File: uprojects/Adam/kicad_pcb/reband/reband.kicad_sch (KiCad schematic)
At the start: 32 parts, among them IC1 USBLC6-2SC6, J1 S2B-ZRLFSN, J2 USB4215-03-A, U1 ESP32-C3FH4, U2 TLV75533PDBVR, U3 MAX30009ENA+T, U4 BQ25100YFPR, U5 BNO055, U7 TCR2EF18_LMCT, Y1 ECS-400-18-33-JGN-TR3

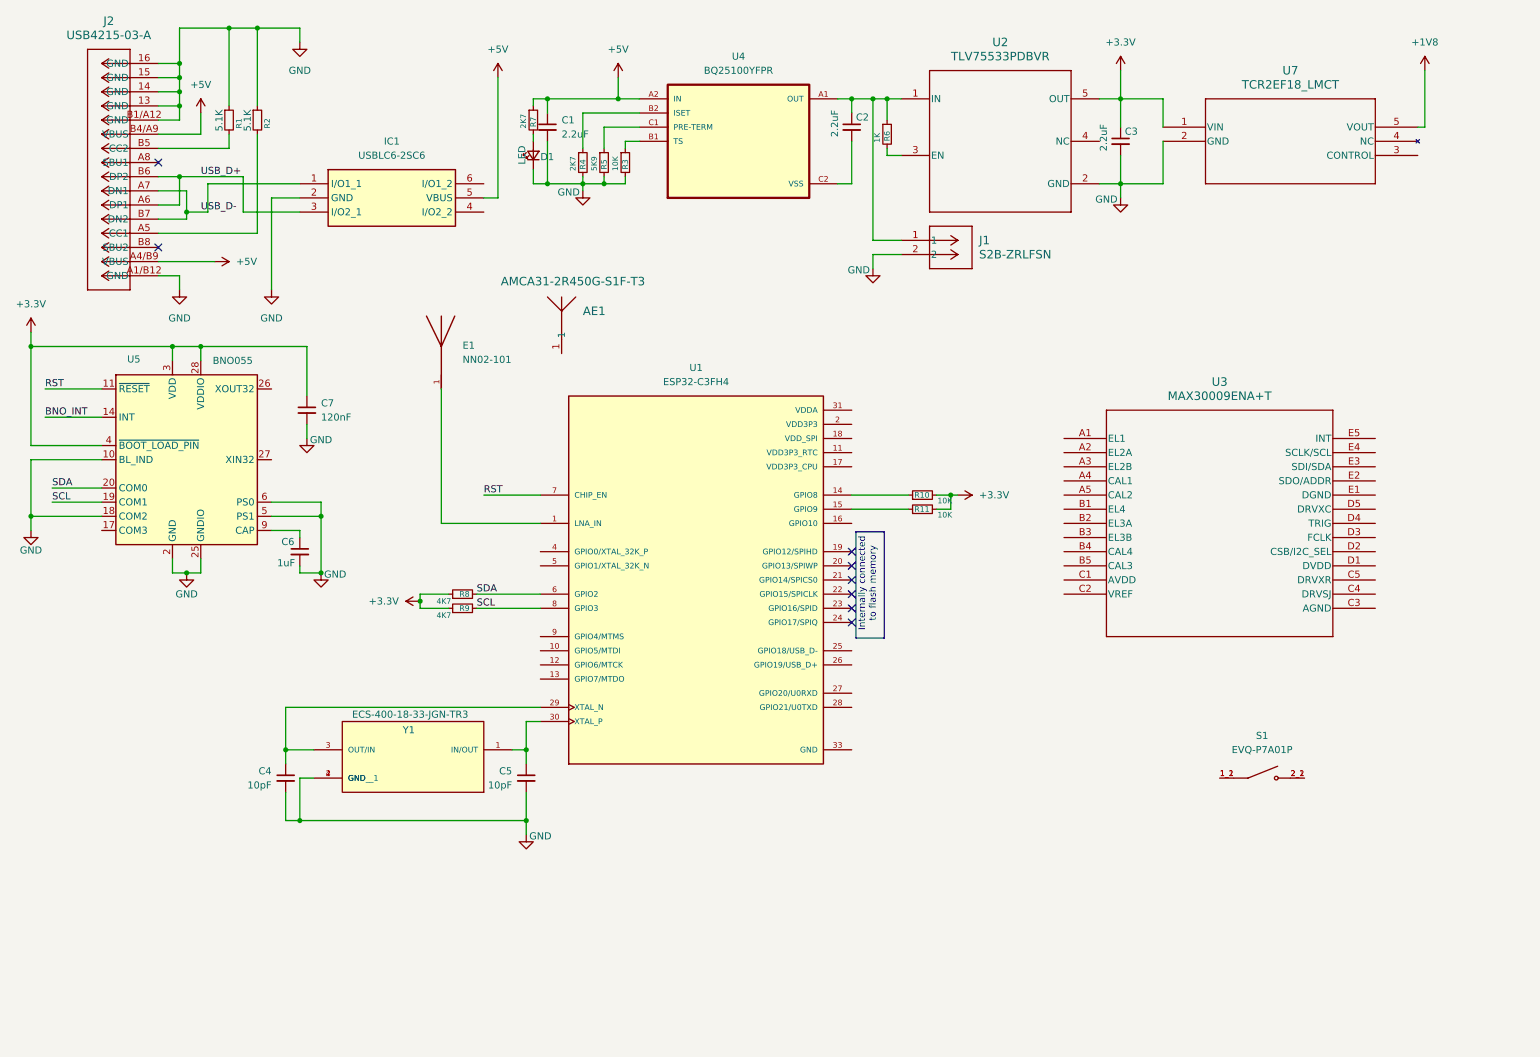
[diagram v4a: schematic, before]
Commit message: Update 29 May 2026
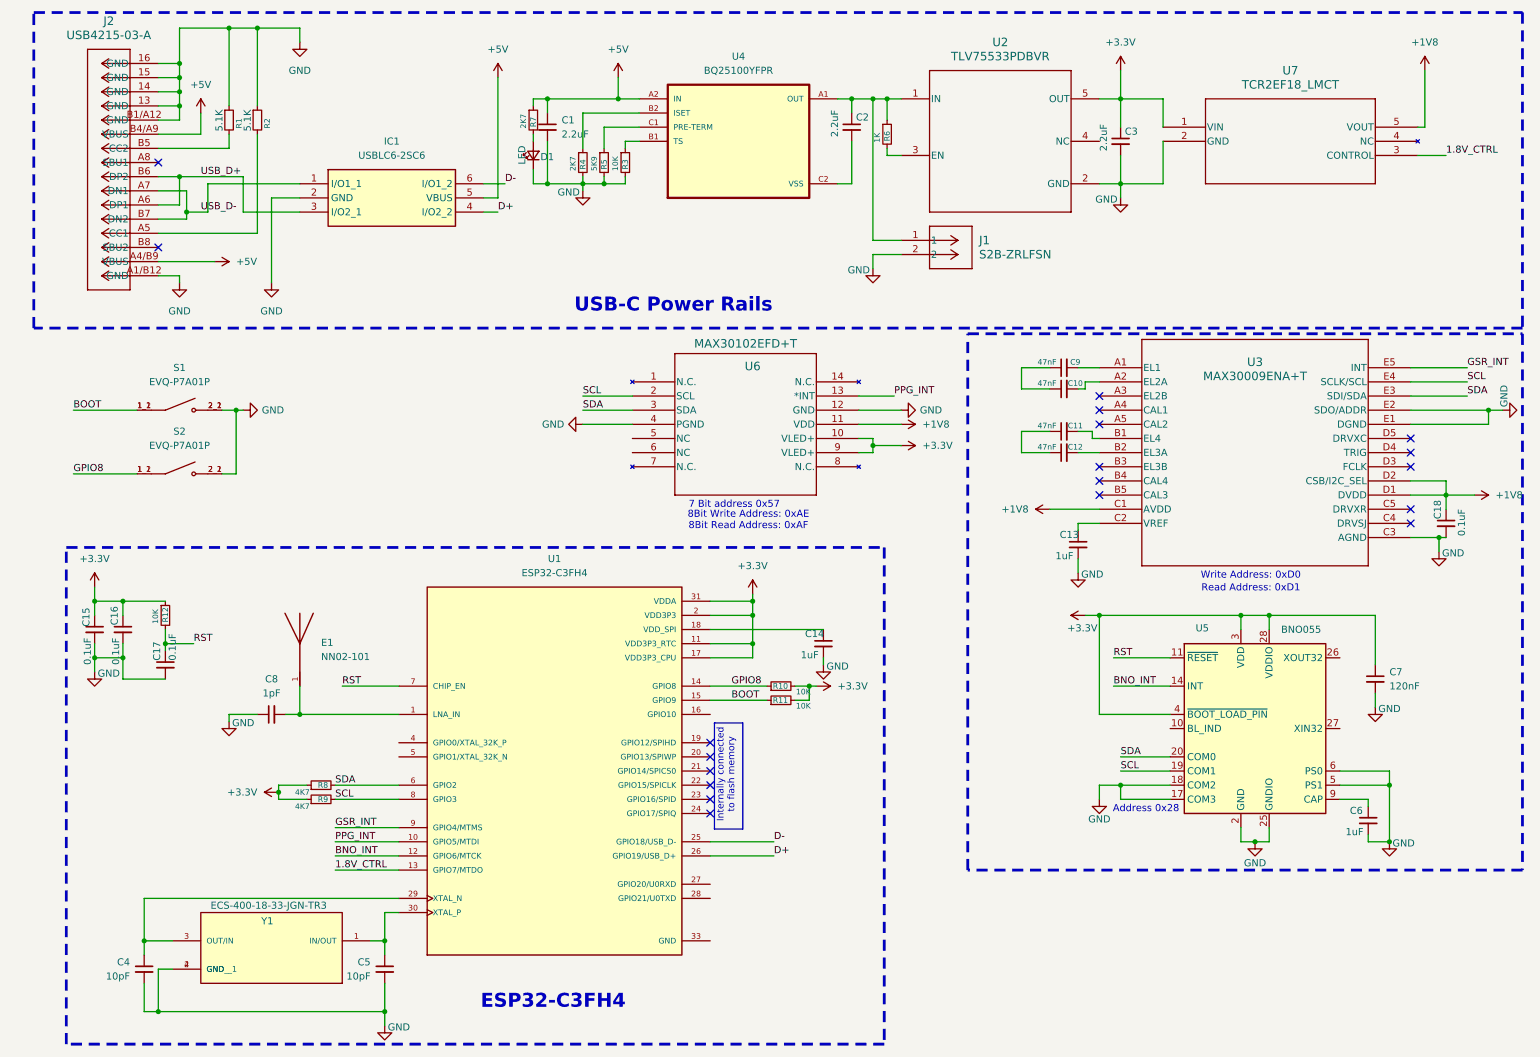
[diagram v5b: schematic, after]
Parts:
- removed AE1: AMCA31-2R450G-S1F-T3, AMCA31_2R450G_S1F_T3:ANT_AMCA31-2R450G-S1F-T3_ABR, symbol AMCA31_2R450G_S1F_T3:AMCA31-2R450G-S1F-T3
- added C10, C11, C12, C9: 47nF, Capacitor_SMD:C_0402_1005Metric_Pad0.74x0.62mm_HandSolder, symbol Device:C_Small
- added C13, C14: 1uF, Capacitor_SMD:C_0402_1005Metric_Pad0.74x0.62mm_HandSolder, symbol Device:C_Small
- added C15, C16, C17, C18: 0.1uF, Capacitor_SMD:C_0402_1005Metric_Pad0.74x0.62mm_HandSolder, symbol Device:C_Small
- added C8: 1pF, Capacitor_SMD:C_0402_1005Metric_Pad0.74x0.62mm_HandSolder, symbol Device:C_Small
- added R12: 10K, Resistor_SMD:R_0402_1005Metric_Pad0.72x0.64mm_HandSolder, symbol Device:R_Small
- added S2: EVQ-P7A01P, EVQ_P7A01P:SW_EVQ-P7A01P, symbol EVQ-P7A01P:EVQ-P7A01P
- added U6: MAX30102EFD+T, MAX30102EFD_T:21-1048_F143A5&plus_1_MXM, symbol MAX30102EFD_T:MAX30102EFD+T
- S1: DigiKey (none) -> P16763TR-ND; Manufacturer_Part_Number (none) -> EVQ-P7A01P
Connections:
- net VDD3P3 is gone; now on net +3.3V: U1.2 (VDD3P3), U1.3 (VDD3P3)
- net VDDA is gone; now on net +3.3V: U1.31 (VDDA), U1.32 (VDDA)
- net +1V8: now also U3.C1 (AVDD), U3.D1 (DVDD), U3.D2 (CSB/I2C_SEL), C18.1, U6.11 (VDD)
- net +3.3V: now also U1.11 (VDD3P3_RTC), U1.17 (VDD3P3_CPU), C15.1, C16.1, R12.1, U6.10 (VLED+), U6.9 (VLED+)
- net BNO_INT: now also U1.12 (GPIO6/MTCK)
- net GND: now also S1.2_1, S1.2_2, U3.C3 (AGND), U3.E1 (DGND), U3.E2 (SDO/ADDR), U5.17 (COM3), C13.2, C14.2, C15.2, C16.2, C17.2, C18.2, C8.1, S2.2_1, S2.2_2, U6.12 (GND), U6.4 (PGND); no longer U5.10 (BL_IND)
- net RST: now also C17.1, R12.2
- net SCL: now also U3.E4 (SCLK/SCL), U6.2 (SCL)
- net SDA: now also U3.E3 (SDI/SDA), U6.3 (SDA)
- net at E1.1, U1.1 (LNA_IN): now also C8.2
- net GPIO8: now reaches R10.1, U1.14 (GPIO8)
- net GPIO8: now also S2.1_1, S2.1_2
- net 1.8V_CTRL: now reaches U7.3 (CONTROL)
- net 1.8V_CTRL: now also U1.13 (GPIO7/MTDO)
- net PPG_INT: now reaches U1.10 (GPIO5/MTDI)
- net PPG_INT: now also U6.13 (*INT)
- net BOOT: now reaches R11.1, U1.15 (GPIO9)
- net BOOT: now also S1.1_1, S1.1_2
- net at U1.18 (VDD_SPI): now also C14.1
- net D-: now reaches U1.25 (GPIO18/USB_D-)
- net D-: now also IC1.6 (I/O1_2)
- net D+: now reaches U1.26 (GPIO19/USB_D+)
- net D+: now also IC1.4 (I/O2_2)
- net GSR_INT: now reaches U1.9 (GPIO4/MTMS)
- net GSR_INT: now also U3.E5 (INT)
- net at U3.A1 (EL1): now also C9.2
- net at U3.A2 (EL2A): now also C10.2
- net at U3.B1 (EL4): now also C11.2
- net at U3.B2 (EL3A): now also C12.2
- net at U3.C2 (VREF): now also C13.1
- new net: C10.1, C9.1
- new net: C11.1, C12.1
- no-connect marks 8 -> 19
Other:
- note added: "7 Bit address 0x57"
- note added: "8Bit Read Address: 0xAF"
- note added: "8Bit Write Address: 0xAE"
- note added: "Address 0x28"
- note added: "ESP32-C3FH4"
- note added: "Read Address: 0xD1"
- note added: "USB-C Power Rails"
- note added: "Write Address: 0xD0"
- moved on the sheet: C4, C5, C6, C7, E1, R10, R11, R8, R9, S1, U1, U3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
